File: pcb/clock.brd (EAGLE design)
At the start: 107.8 x 42.2 mm, 50 parts, among them K1 JS-M1-9V-4, K2 JS-M1-9V-4, Q1 BC447, Q2 BC447, Q3 BC447, Q4 BC447, Q5 BC447, Q6 BC447, Q8 CSM-7X-DU, Q9 MC-306, U1 ATMEGA328P-AU, U2 PCF8563T/F4

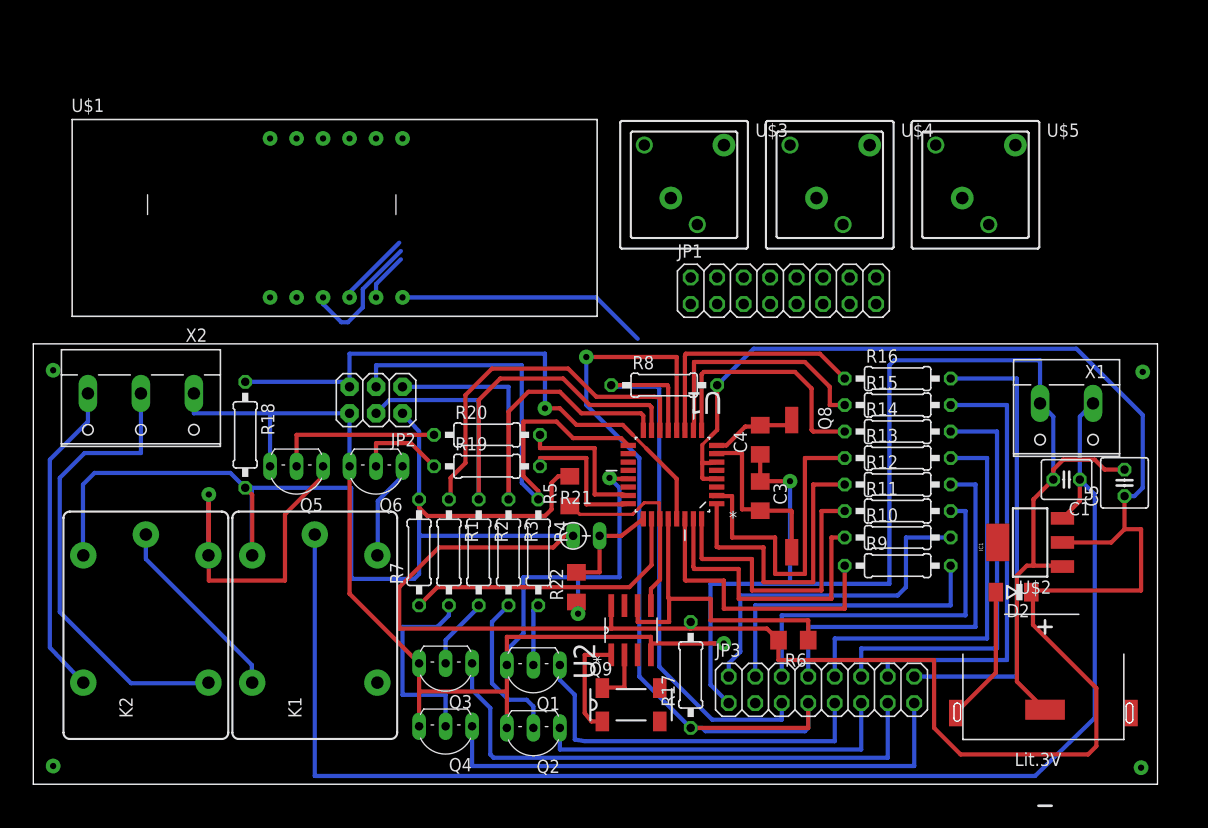
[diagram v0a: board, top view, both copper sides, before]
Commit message: some small things
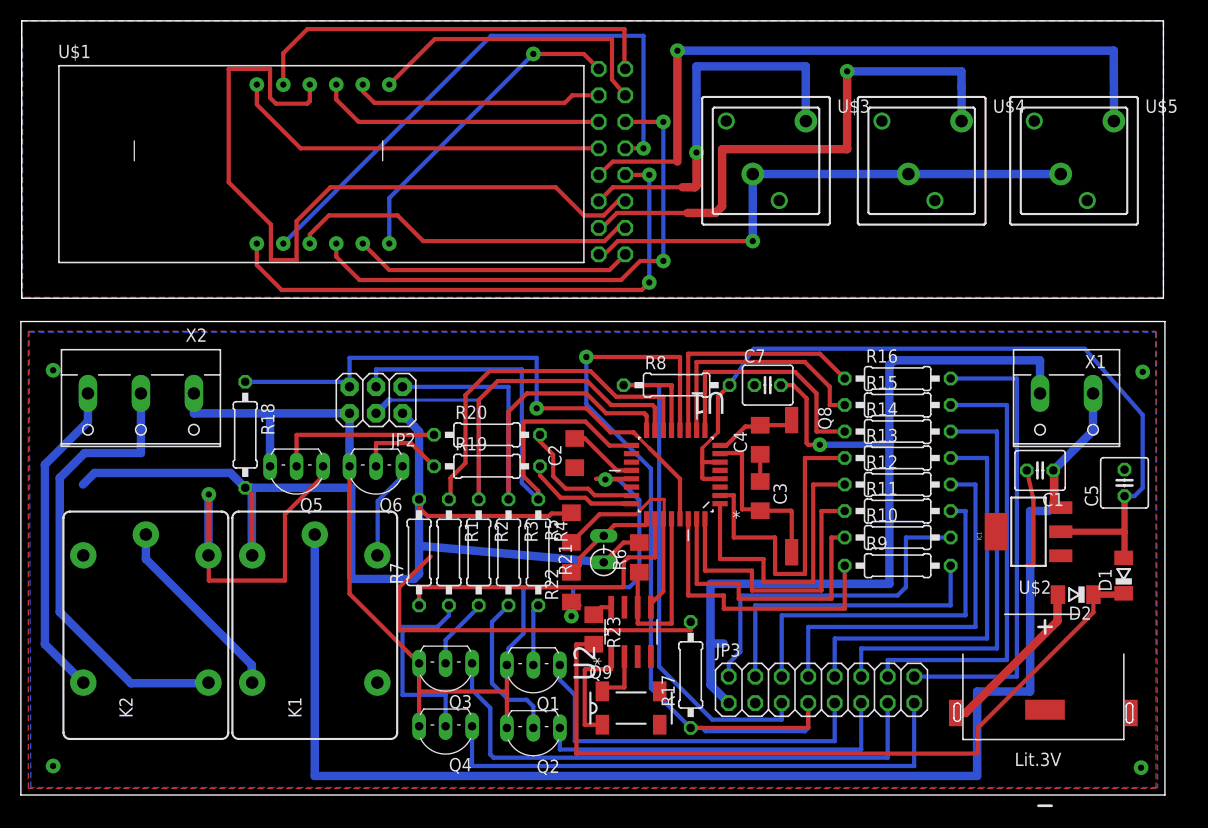
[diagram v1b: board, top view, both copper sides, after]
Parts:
- added C2: (no value), rcl:C1206
- added C7: (no value), rcl:C025-040X050
- added D1: (no value), diode:SOD80C
- added R23: (no value), rcl:R1206
- moved JP1 20.6 mm to (51.8, 59.7), flipped to the bottom, turned to 90 degrees
- moved R6 16.8 mm to (54.5, 21.7), turned to 90 degrees
- moved U$5 9.72 mm to (94.9, 58.5)
- moved U$4 9.11 mm to (80.2, 58.5)
- moved U$3 8.19 mm to (65.3, 58.5)
- moved D2 5.96 mm to (96.3, 18.2)
- moved U$1 5.31 mm to (3.81, 57.5)
- moved R5 3.50 mm to (47.9, 24.6)
- moved C1 2.69 mm to (92.9, 30.1)
- moved R21 2.10 mm to (51.0, 22.5), turned to 90 degrees
- moved R8 1.19 mm to (58.0, 38.3)
- moved IC1 1.04 mm to (91.8, 24.2)
- moved X1 0.95 mm to (95.4, 36.8)
- moved R22 0.48 mm to (47.9, 18.9)
- moved U1 0.32 mm to (57.9, 29.7)
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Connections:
- removed net AVCC: U1.18
- new net N$66: C2.2, U1.20
- new net N$67: D1.C, D2.C, R23.2
- new net N$68: R23.1, U2.8
- net GND: now also C2.1, C7.2
- net VCC: now also C7.1, D1.A, U1.18; no longer D2.C, U2.8
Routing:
- net VCC: track 325.8 -> 225.8 mm
- net N$67: track 0.00 -> 73.7 mm
- net N$52: track 0.00 -> 73.2 mm
- net N$51: track 0.00 -> 67.3 mm, vias 0 -> 1
- net N$54: track 0.00 -> 55.3 mm, vias 0 -> 1
- net N$55: track 0.00 -> 53.6 mm, vias 0 -> 2
- net N$49: track 0.00 -> 53.3 mm, vias 0 -> 1
- net N$53: track 7.21 -> 51.3 mm, vias 0 -> 2
- net N$32: track 0.00 -> 40.5 mm
- net N$50: track 0.00 -> 37.1 mm, vias 0 -> 1
- net N$58: track 0.00 -> 36.4 mm
- net N$44: track 0.00 -> 29.0 mm
- net N$59: track 0.00 -> 27.5 mm
- net N$60: track 0.00 -> 24.0 mm
- net N$56: track 4.64 -> 26.8 mm
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- added copper zone on layer 1, net GND
- added copper zone on layer 16, net GND
- added copper zone on layer 16, net VCC
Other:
- board size 107.8 x 42.2 mm -> 109.7 x 74.2 mm
